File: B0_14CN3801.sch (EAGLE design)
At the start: 1 part

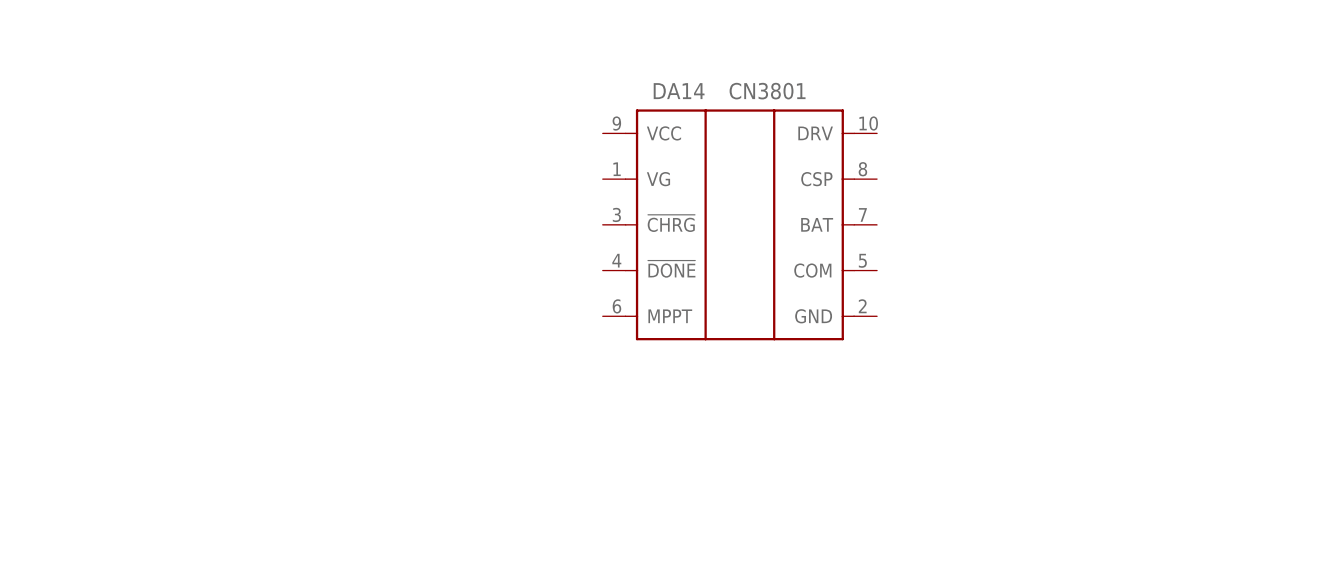
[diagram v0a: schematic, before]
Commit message: .
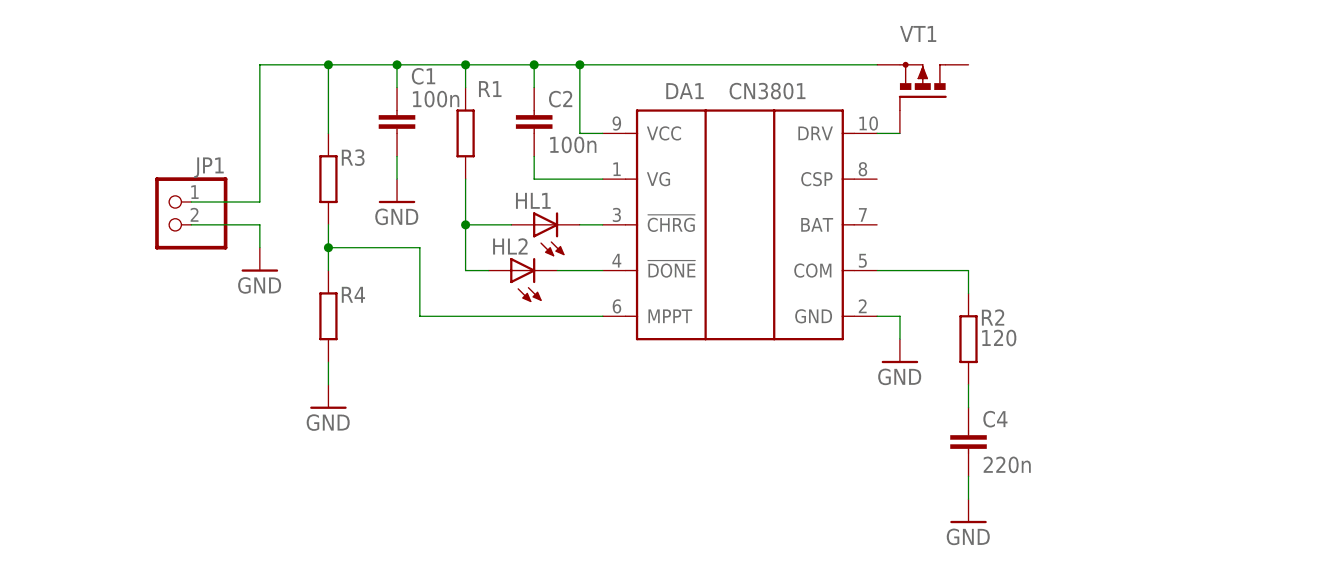
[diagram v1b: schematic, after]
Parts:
- added C1, C2: 100n, rcl:C-EUC0805
- added C4: 220n, rcl:C-EUC0805
- added HL1, HL2: (no value), led:LEDCHIPLED_0603
- added JP1: (no value), Разъёмы штырьковые 2.54мм:PINHD-1X2/2
- added R1, R3, R4: (no value), rcl:R-EU_R0805
- added R2: 120, rcl:R-EU_R0805
- added VT1: (no value), m_transistor:MOSFET-P_TO220_V
- renumbered DA14 to DA1
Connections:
- new net GND: C1.2, C4.2, DA1.GND, JP1.2, R4.1
- new net N$1: C1.1, C2.1, DA1.VCC, JP1.1, R1.2, R3.2, VT1.S
- new net N$2: C2.2, DA1.VG
- new net N$3: DA1.MPPT, R3.1, R4.2
- new net N$4: DA1.COM, R2.2
- new net N$5: HL1.A, HL2.A, R1.1
- new net N$6: DA1.!CHRG, HL1.C
- new net N$7: DA1.!DONE, HL2.C
- new net N$8: C4.1, R2.1
- new net N$9: DA1.DRV, VT1.G

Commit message: .
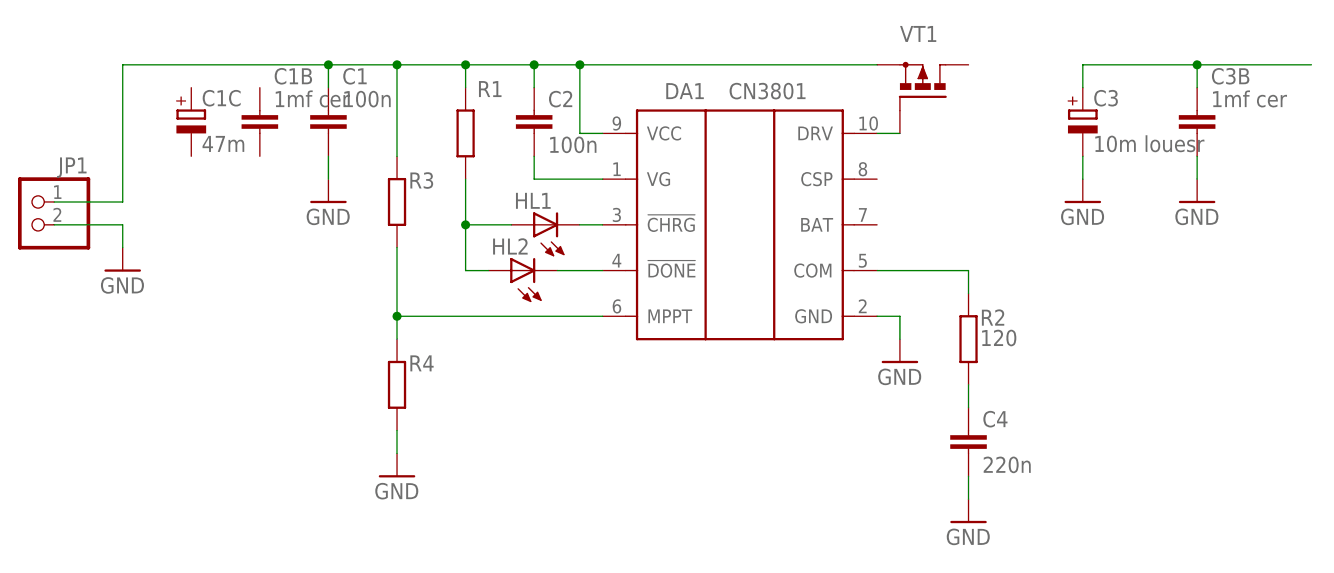
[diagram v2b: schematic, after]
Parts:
- added C1B, C3B: 1mf cer, rcl:C-EUC0805
- added C1C: 47m, rcl:CPOL-EUE2.5-6
- added C3: 10m louesr, rcl:CPOL-EUE2.5-6
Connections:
- new net N$10: C3.+, C3B.1
- net GND: now also C3.-, C3B.2
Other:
- note added: "1.205v max"
- moved on the sheet: C1, JP1, R3, R4
